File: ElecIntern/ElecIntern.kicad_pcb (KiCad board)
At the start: 2 copper layers, 70 x 70 mm, 22 parts, among them J1 Conn_01x02, J2 Conn_Servo, J3 Conn_01x05, J4 Conn_01x05, U1 MR45V200B, U3 PMOS, U4 R-78C5.0-1.0, U5 R-78C3.3-1.0, U7 TEENSY3.2, U8 Xbee802.15.4, U9 MPU-6050

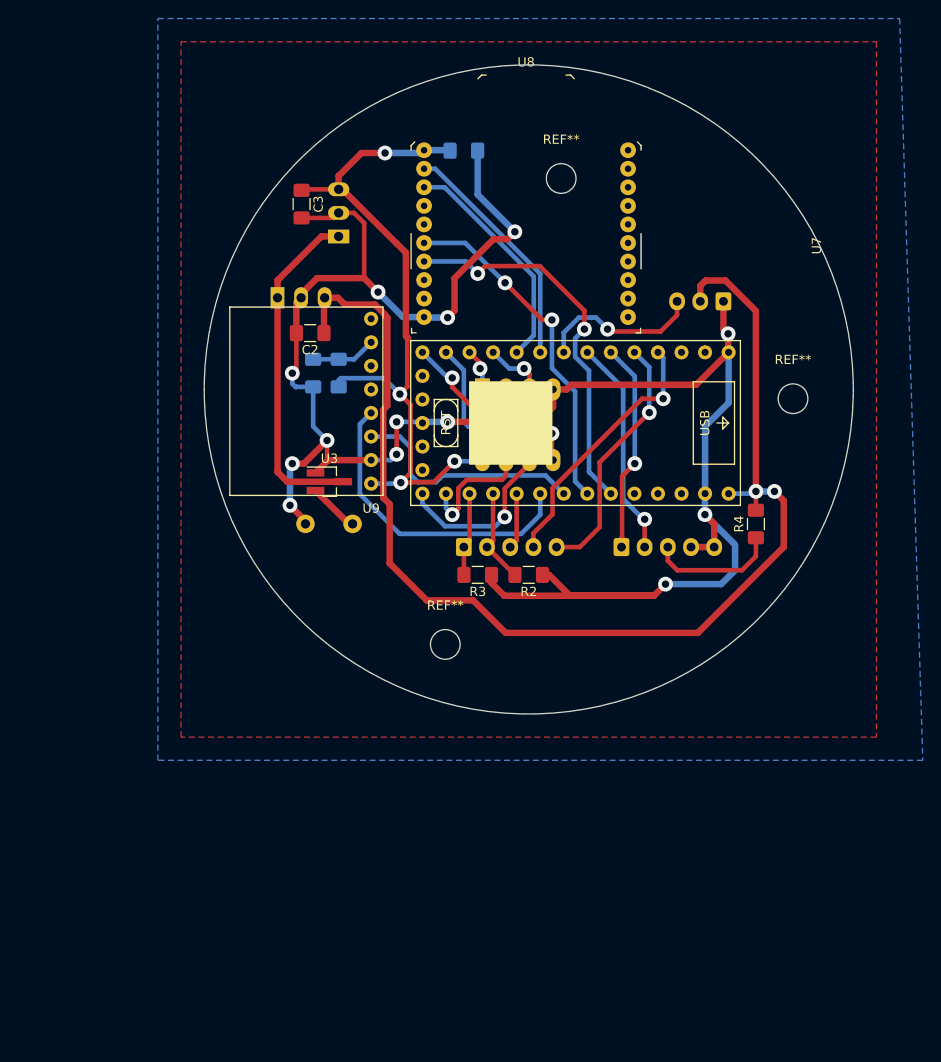
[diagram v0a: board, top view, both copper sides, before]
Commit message: Grosse mise à jour
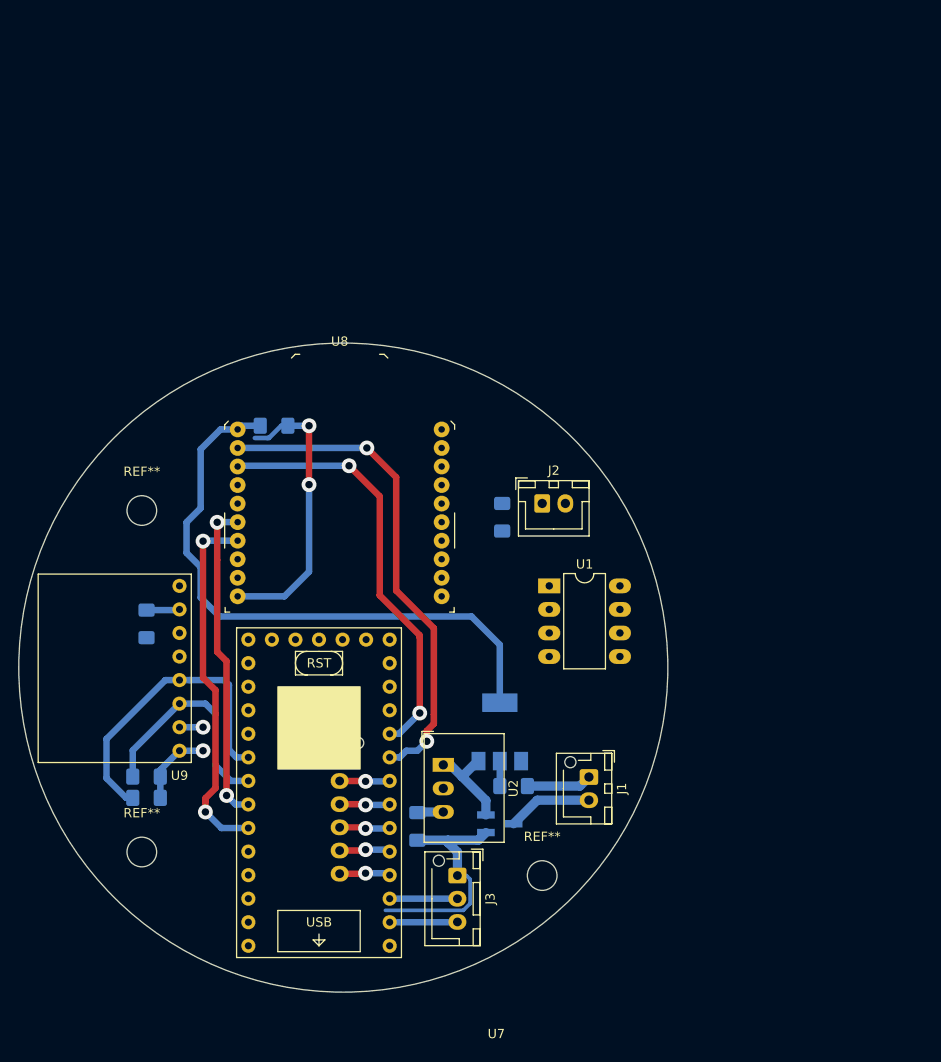
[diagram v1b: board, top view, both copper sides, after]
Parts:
- removed C2: 10uF 1206, Capacitor_SMD:C_1206_3216Metric_Pad1.42x1.75mm_HandSolder
- removed JP1: SolderJumper_2_Open, Resistor_SMD:R_1206_3216Metric_Pad1.42x1.75mm_HandSolder
- removed the REF** at (161.0, 97.5)
- removed the REF** at (173.5, 47.2)
- removed the REF** at (198.5, 71.0)
- removed U5: R-78C3.3-1.0, Converter_DCDC:Converter_DCDC_RECOM_R-78E-0.5_THT
- added C1: 10uF 1206, Capacitor_SMD:C_1206_3216Metric_Pad1.42x1.75mm_HandSolder, B.Cu at (158.0, 117.1)
- added REF**: MountingHole_3.2mm_M3, MountingHole:MountingHole_3.2mm_M3, F.Cu at (171.4, 122.4)
- added REF**: MountingHole_3.2mm_M3, MountingHole:MountingHole_3.2mm_M3, F.Cu at (128.3, 119.9)
- added REF**: MountingHole_3.2mm_M3, MountingHole:MountingHole_3.2mm_M3, F.Cu at (128.3, 83.1)
- added U2: R-78C5.0-1.0, Converter_DCDC:Converter_DCDC_RECOM_R-78E-0.5_THT, F.Cu at (160.8, 110.5)
- C3, R4, U3: moved to B.Cu
- J1: footprint rex:BatConn -> Connector_JST:JST_XH_B2B-XH-AM_1x02_P2.50mm_Vertical; moved to F.Cu
- J2: value Conn_Servo -> Conn_01x02; footprint Connector_JST:JST_XH_B3B-XH-A_1x03_P2.50mm_Vertical -> Connector_JST:JST_XH_B2B-XH-A_1x02_P2.50mm_Vertical; moved to F.Cu
- J3: value Conn_01x05 -> Conn_01x03; footprint Connector_JST:JST_XH_B5B-XH-A_1x05_P2.50mm_Vertical -> Connector_JST:JST_XH_B3B-XH-AM_1x03_P2.50mm_Vertical; moved to F.Cu
- J4: value Conn_01x05 -> Conn_01x06; footprint Connector_JST:JST_XH_B5B-XH-A_1x05_P2.50mm_Vertical -> Connector_JST:JST_XH_B6B-XH-AM_1x06_P2.50mm_Vertical
- R2, R3: value 1kR-pulldown -> R; moved to B.Cu
- U1: moved to F.Cu
- U4: value R-78C5.0-1.0 -> AMS1117-3.3; footprint Converter_DCDC:Converter_DCDC_RECOM_R-78E-0.5_THT -> Package_TO_SOT_SMD:SOT-223-3_TabPin2
- moved U7 73.7 mm to (155.0, 130.0), turned to 180 degrees
- moved C3 66.8 mm to (168.4, 112.8), turned to 0 degrees
- moved U4 52.6 mm to (166.9, 106.9), turned to 90 degrees
- moved R2 46.6 mm to (128.8, 111.8)
- moved R3 43.1 mm to (128.8, 114.0)
- moved U3 41.2 mm to (166.9, 116.8)
- moved J1 39.1 mm to (176.5, 111.8), turned to 270 degrees
- moved J4 38.0 mm to (149.6, 109.7), turned to 270 degrees
- moved U8 36.2 mm to (149.6, 83.3)
- moved C4 36.0 mm to (142.5, 73.9)
- moved U9 35.5 mm to (132.3, 109.0)
- moved J3 35.4 mm to (162.3, 122.4), turned to 270 degrees
- moved R1 32.5 mm to (128.8, 95.3)
- moved J2 29.3 mm to (171.4, 82.3), turned to 0 degrees
- moved R4 27.4 mm to (167.1, 83.8), turned to 270 degrees
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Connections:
- J2 pad 1: GND -> /LED_POWER
- J2 pad 2: +5V -> GND
- J3 pad 1: /lectureTrappe -> GND
- J3 pad 2: /lectureArmement -> /TX1_Teensy
- J3 pad 3: /ecritureArmement -> /RX1_Teensy
- J4 pad 1: /LED3 -> GND
- J4 pad 2: /LED4 -> /io5
- J4 pad 3: /LED_POWER -> /io4
- J4 pad 4: GND -> /io3
- J4 pad 5: GND -> /io2
- R2 pad 1: GND -> +3V3
- R2 pad 2: /lectureArmement -> /SCL
- R3 pad 1: GND -> +3V3
- R3 pad 2: /lectureTrappe -> /SDA
- U4 pad 1: +12V -> GND
- U4 pad 2: GND -> +3V3
- U4 pad 3: +5V -> +12V
- U7 pad 17: /lectureTrappe -> Net-(U7-Pad17)
- U7 pad 18: /lectureArmement -> Net-(U7-Pad18)
- U7 pad 19: /ecritureArmement -> Net-(U7-Pad19)
- U7 pad 2: Net-(U7-Pad2) -> /RX1_Teensy
- U7 pad 3: Net-(U7-Pad3) -> /TX1_Teensy
- U7 pad 4: /LED1 -> /io1
- U7 pad 5: /LED2 -> /io2
- U7 pad 6: /LED3 -> /io3
- U7 pad 7: /LED4 -> /io4
- U7 pad 8: /PWM_Servo -> /io5
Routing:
- net GND: track 221.4 -> 66.1 mm, vias 13 -> 3
- net +5V: track 130.6 -> 2.82 mm, vias 2 -> 0
- net /LED1: track 28.4 -> 0.00 mm, vias 1 -> 0
- net /RX_Teensy: track 25.7 -> 53.6 mm, vias 0 -> 2
- net /LED2: track 27.3 -> 0.00 mm, vias 1 -> 0
- net +12V: track 36.7 -> 10.2 mm
- net /LED4: track 23.6 -> 0.00 mm, vias 1 -> 0
- net /LED3: track 22.7 -> 0.00 mm, vias 1 -> 0
- net /TX_Teensy: track 24.8 -> 46.0 mm, vias 0 -> 2
- net /MOSI: track 21.2 -> 0.00 mm, vias 1 -> 0
- net /SCK: track 18.6 -> 0.00 mm, vias 1 -> 0
- net /PWM_Servo: track 17.9 -> 0.00 mm, vias 1 -> 0
- net /MISO: track 14.1 -> 0.00 mm, vias 1 -> 0
- net /LED_POWER: track 14.0 -> 0.00 mm
- net /~Hold~_FRAM: track 13.0 -> 0.00 mm, vias 1 -> 0
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- removed copper zone on B.Cu, net GND
- removed copper zone on F.Cu, net GND
